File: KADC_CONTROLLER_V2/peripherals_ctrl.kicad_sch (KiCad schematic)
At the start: 82 parts

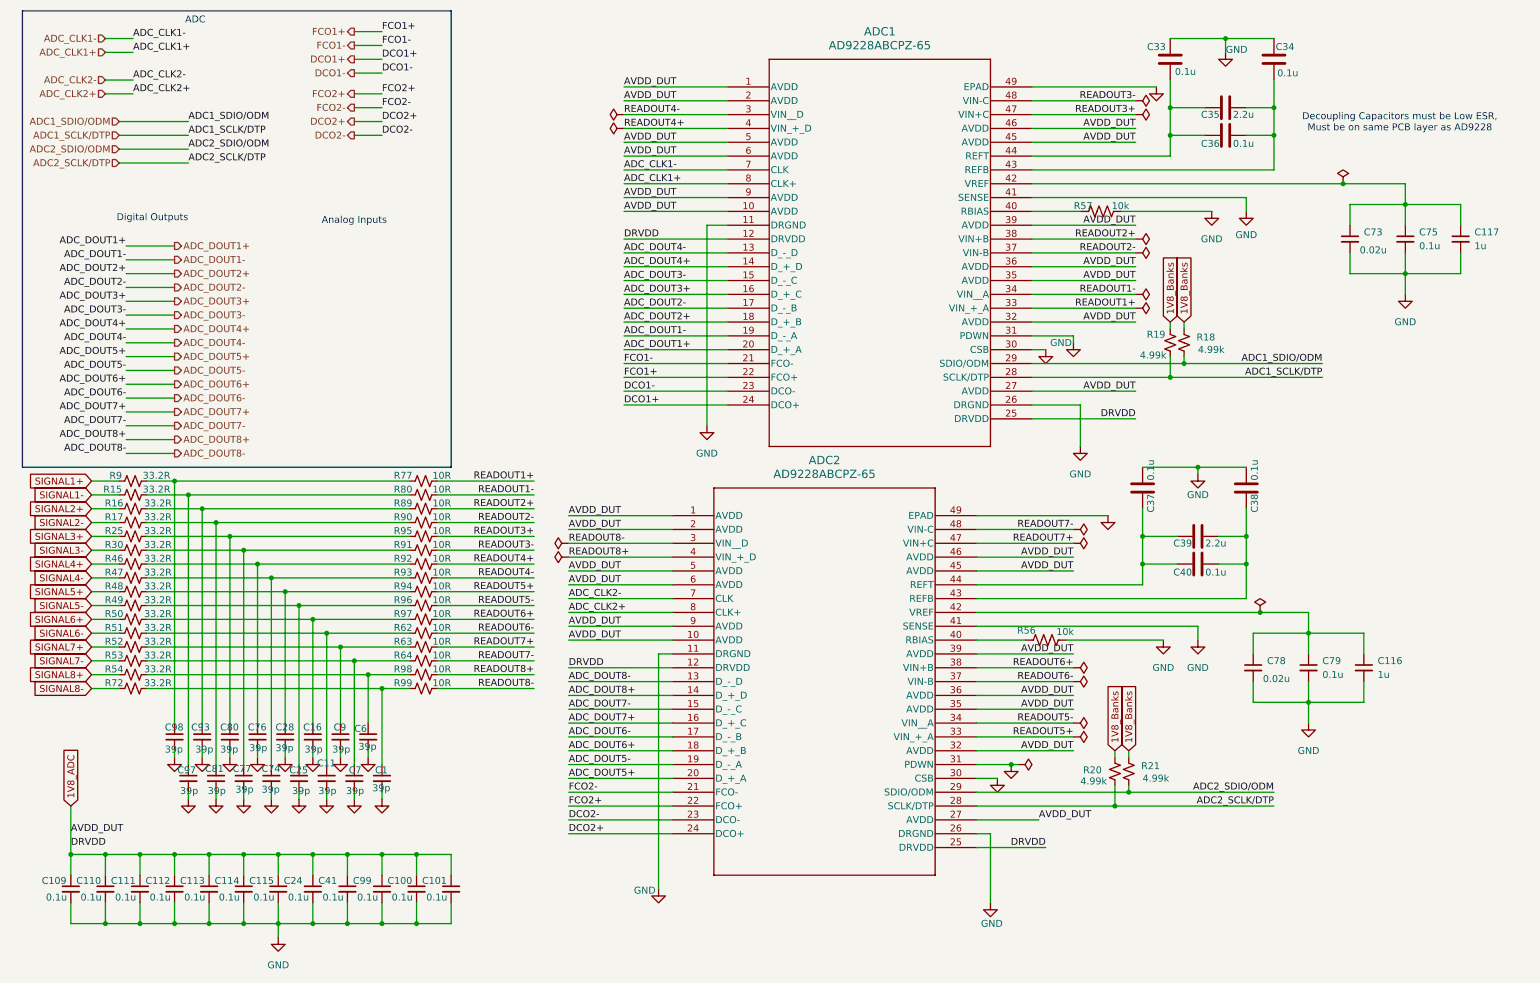
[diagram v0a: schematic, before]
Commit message: Reupdate for verify
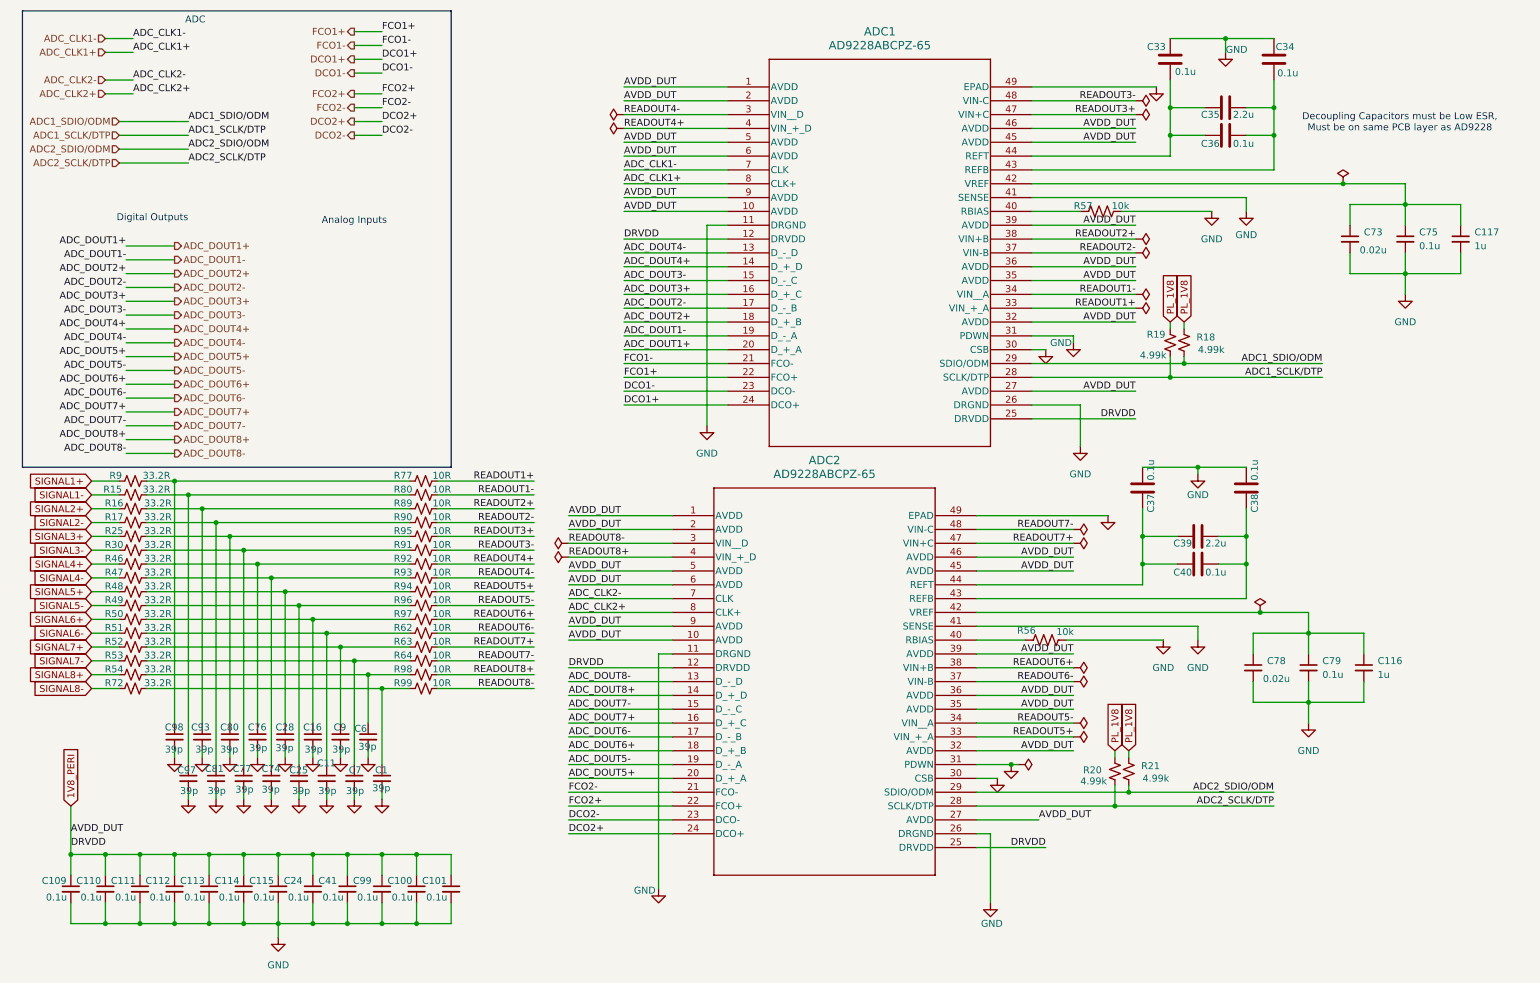
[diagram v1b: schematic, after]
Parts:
- ADC1, ADC2: footprint CP_48_8_ADI -> AD9228ABCPZ_65:CP_48_8_ADI
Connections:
- net 1V8_ADC renamed 1V8_PERI
- net 1V8_Banks renamed PL_1V8
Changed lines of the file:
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@@
 		)
 	)
-	(global_label "1V8_Banks"
+	(global_label "PL_1V8"
 		(shape input)
 		(at 215.9 148.59 90)
@@
 		)
 		(property "Intersheetrefs" "${INTERSHEET_REFS}"
-			(at 215.9 135.5054 90)
+			(at 215.9 138.8315 90)
 			(hide yes)
 			(show_name no)
@@
 		)
 	)
-	(global_label "1V8_Banks"
+	(global_label "PL_1V8"
 		(shape input)
 		(at 223.52 69.85 90)
@@
 		)
 		(property "Intersheetrefs" "${INTERSHEET_REFS}"
-			(at 223.52 56.7654 90)
+			(at 223.52 60.0915 90)
 			(hide yes)
 			(show_name no)
@@
 		)
 	)
-	(global_label "1V8_Banks"
+	(global_label "PL_1V8"
 		(shape input)
 		(at 213.36 148.59 90)
@@
 		)
 		(property "Intersheetrefs" "${INTERSHEET_REFS}"
-			(at 213.36 135.5054 90)
+			(at 213.36 138.8315 90)
 			(hide yes)
 			(show_name no)
@@
 		)
 	)
-	(global_label "1V8_ADC"
+	(global_label "1V8_PERI"
 		(shape input)
 		(at 21.59 158.75 90)
@@
 		)
 		(property "Intersheetrefs" "${INTERSHEET_REFS}"
-			(at 21.59 147.661 90)
+			(at 21.59 146.9958 90)
 			(hide yes)
 			(show_name no)
@@
 		)
 	)
-	(global_label "1V8_Banks"
+	(global_label "PL_1V8"
 		(shape input)
 		(at 226.06 69.85 90)
@@
 		)
 		(property "Intersheetrefs" "${INTERSHEET_REFS}"
-			(at 226.06 56.7654 90)
+			(at 226.06 60.0915 90)
 			(hide yes)
 			(show_name no)
@@
 			)
 		)
-		(property "Footprint" "CP_48_8_ADI"
+		(property "Footprint" "AD9228ABCPZ_65:CP_48_8_ADI"
 			(at 168.402 8.636 0)
 			(hide yes)
@@
 			)
 		)
-		(property "Footprint" "CP_48_8_ADI"
+		(property "Footprint" "AD9228ABCPZ_65:CP_48_8_ADI"
 			(at 158.242 87.376 0)
 			(hide yes)
